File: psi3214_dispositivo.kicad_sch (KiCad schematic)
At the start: 0 parts

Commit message: Breadboard
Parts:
- added C2: 100n, symbol Device:C
- added C3: 10n, symbol Device:C
- added R11: 27k, symbol Device:R
- added R13, R4: 10k, symbol Device:R
- added R3: 50, symbol Device:R
- added R5: 47k, symbol Device:R
- added R6: 100k, symbol Device:R
- added R7: 63.6k, symbol Device:R
- added R8: 2030, symbol Device:R
- added R9: 6.8k, symbol Device:R
- added U1: TL072, symbol Amplifier_Operational:TL072
- added V1: 1 ac=1, symbol Simulation_SPICE:VDC
- added V2, V3: 9, symbol Simulation_SPICE:VDC
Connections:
- new net: R11.2, R9.2, U1.6 (-)
- new net: C2.1, R3.1
- new net: R3.2, V1.1
- new net: C3.1, R6.1, R7.1, U1.1
- new net: C3.2, R7.2, R8.2, U1.5 (+)
- new net: C2.2, R4.2, U1.3 (+)
- new net: R5.2, R6.2, U1.2 (-)
- new net +9V: U1.8 (V+), V2.1
- new net -9V: U1.4 (V-), V3.2
- new net 0: R13.2, R4.1, R5.1, R8.1, R9.1, V1.2, V2.2, V3.1
- new net out_general: R11.1, R13.1, U1.7

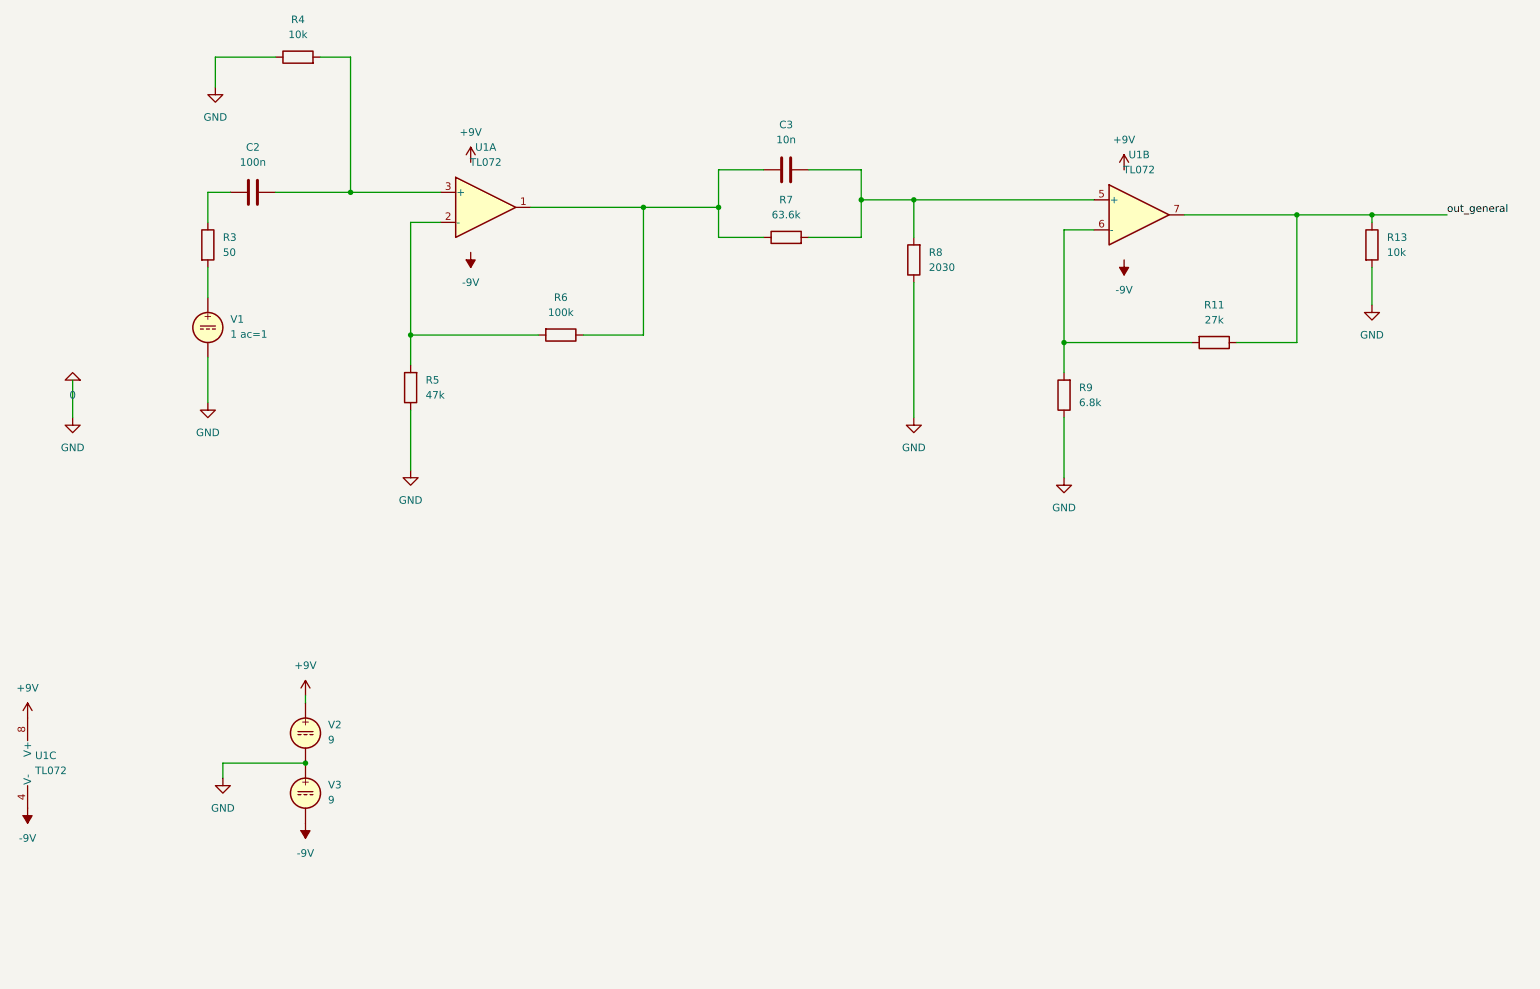
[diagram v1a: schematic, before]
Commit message: Spice Sim working
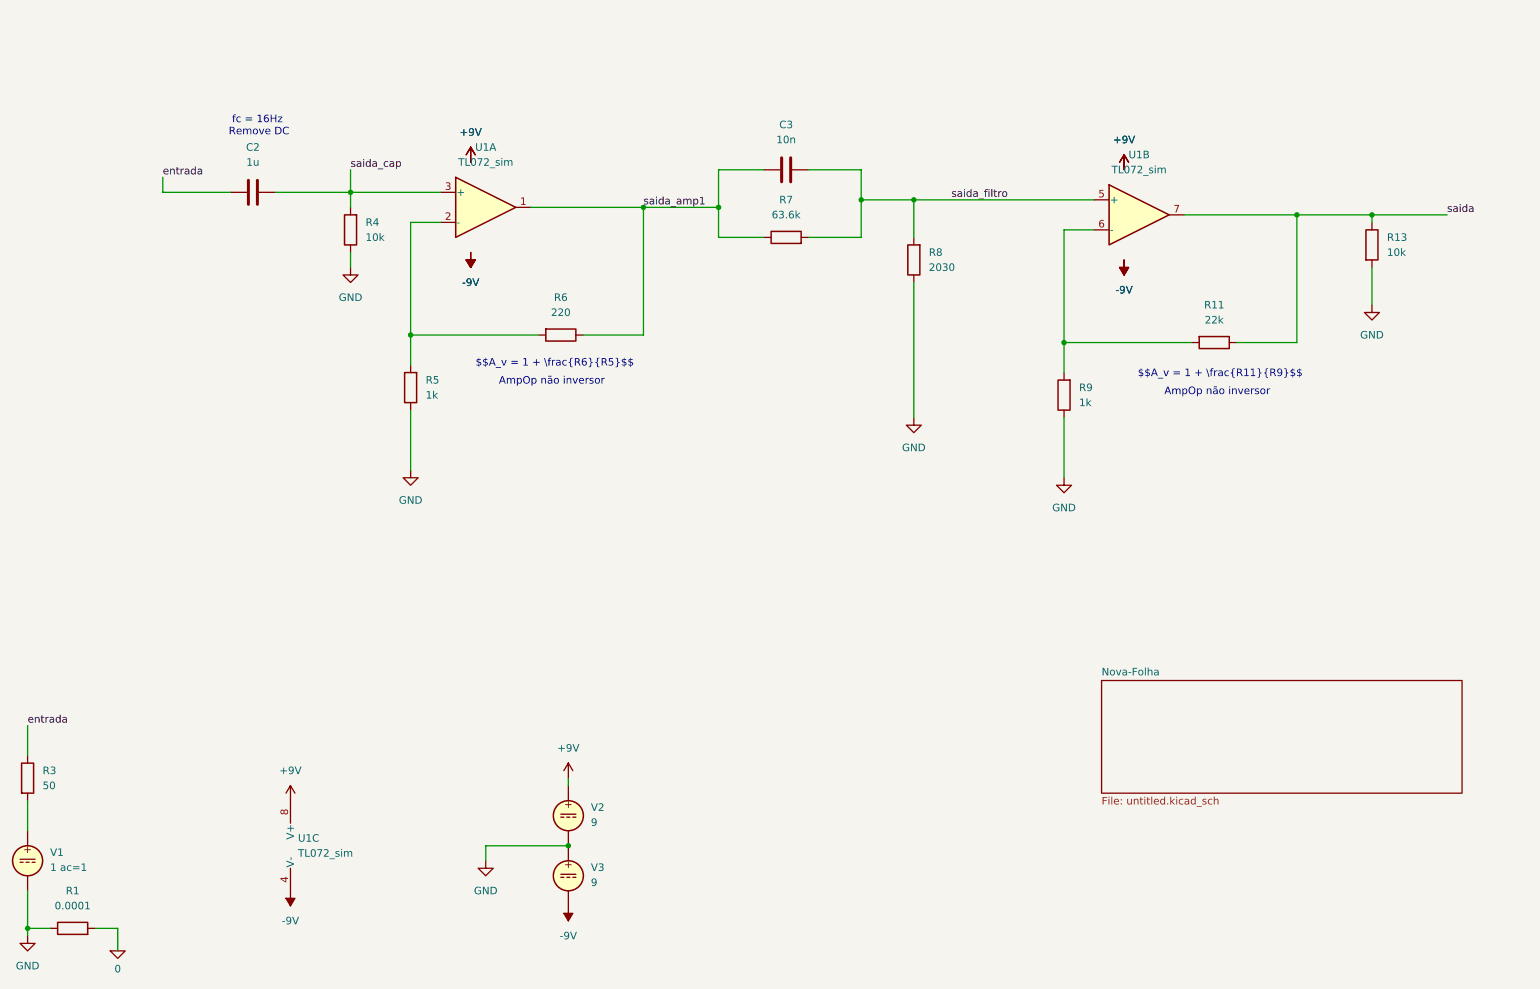
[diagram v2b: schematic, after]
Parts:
- removed U1: TL072, symbol Amplifier_Operational:TL072
- added R1: 0.0001, symbol Device:R
- added U1: TL072_sim, symbol custom:TL072_sim
- C2: value 100n -> 1u
- R11: value 27k -> 22k
- R5: value 47k -> 1k
- R6: value 100k -> 220
- R9: value 6.8k -> 1k
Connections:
- net +9V: now also U1.8 (V+)
- net -9V: now also U1.4 (V-)
- net 0: now also R1.2; no longer R13.2, R4.1, R5.1, R8.1, R9.1, V1.2, V2.2, V3.1
- net at R11.2, R9.2: now also U1.6 (-)
- net entrada: now reaches C2.1, R3.1
- net saida_amp1: now reaches C3.1, R6.1, R7.1
- net saida_amp1: now also U1.1
- net saida_filtro: now reaches C3.2, R7.2, R8.2
- net saida_filtro: now also U1.5 (+)
- net saida_cap: now reaches C2.2, R4.2
- net saida_cap: now also U1.3 (+)
- net at R5.2, R6.2: now also U1.2 (-)
- net out_general renamed saida
- net saida: now also U1.7
- new net GND: R1.1, R13.2, R4.1, R5.1, R8.1, R9.1, V1.2, V2.2, V3.1
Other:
- added sheet Nova-Folha (untitled.kicad_sch)
- note added: "$$A_v = 1 + \frac{R11}{R9}$$"
- note added: "$$A_v = 1 + \frac{R6}{R5}$$"
- note added: "AmpOp não inversor"
- note added: "fc = 16Hz Remove DC"
- moved on the sheet: V2, V3
